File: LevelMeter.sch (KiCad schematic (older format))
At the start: 28 parts, among them U10 NJM4580CG, U8 NJM4580CG, U9 NJM4580CG

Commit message: 改版中
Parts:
- removed C32, C33, C34: 0.1u, Capacitor_SMD:C_0603_1608Metric_Pad1.05x0.95mm_HandSolder, symbol Device:C_Small
- removed C35, C47: 0.47u, Capacitor_THT:CP_Radial_D5.0mm_P2.00mm, symbol Device:CP_Small
- removed C48, C49: option_footprint, Capacitor_SMD:C_0603_1608Metric_Pad1.05x0.95mm_HandSolder, symbol Device:C_Small
- removed D10, D12: SS2040, Diode_SMD:D_SOD-123, symbol Device:D
- removed D11, D13: LED_RED, LED_SMD:LED_0603_1608Metric_Pad1.05x0.95mm_HandSolder, symbol Device:LED
- removed R24: 470k, Resistor_SMD:R_0603_1608Metric_Pad1.05x0.95mm_HandSolder, symbol Device:R_Small
- removed R36: 470, Resistor_SMD:R_0603_1608Metric_Pad1.05x0.95mm_HandSolder, symbol Device:R_Small
- removed unit 3 of U10
- removed unit 2 of U9
- removed unit 1 of U9
- added D10: LED_ORANGE, LED_SMD:LED_0603_1608Metric_Pad1.05x0.95mm_HandSolder, symbol Device:LED
- added D13, D14: 1N4148, Diode_SMD:D_SOD-123, symbol Device:D
- added R23: 1.2k, Resistor_SMD:R_0603_1608Metric_Pad1.05x0.95mm_HandSolder, symbol Device:R_Small
- D8, D9: value SS2040 -> 1N4148
- R21: value 470k -> 22k
- R31: value 4.7k -> 22k
- R32: value 4.7k -> 1.2k
- R35: value 470 -> 1k
- renumbered U10 to U9
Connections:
- wire segments 125 -> 71
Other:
- note added: "-10dBV"
- note removed: "220ms"
- note removed: "Peak\n1/2 Vcc"
- moved on the sheet: C26, C27, C28, C29, C30, C31, R31, R32, R35, U8C, U9A, U9B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

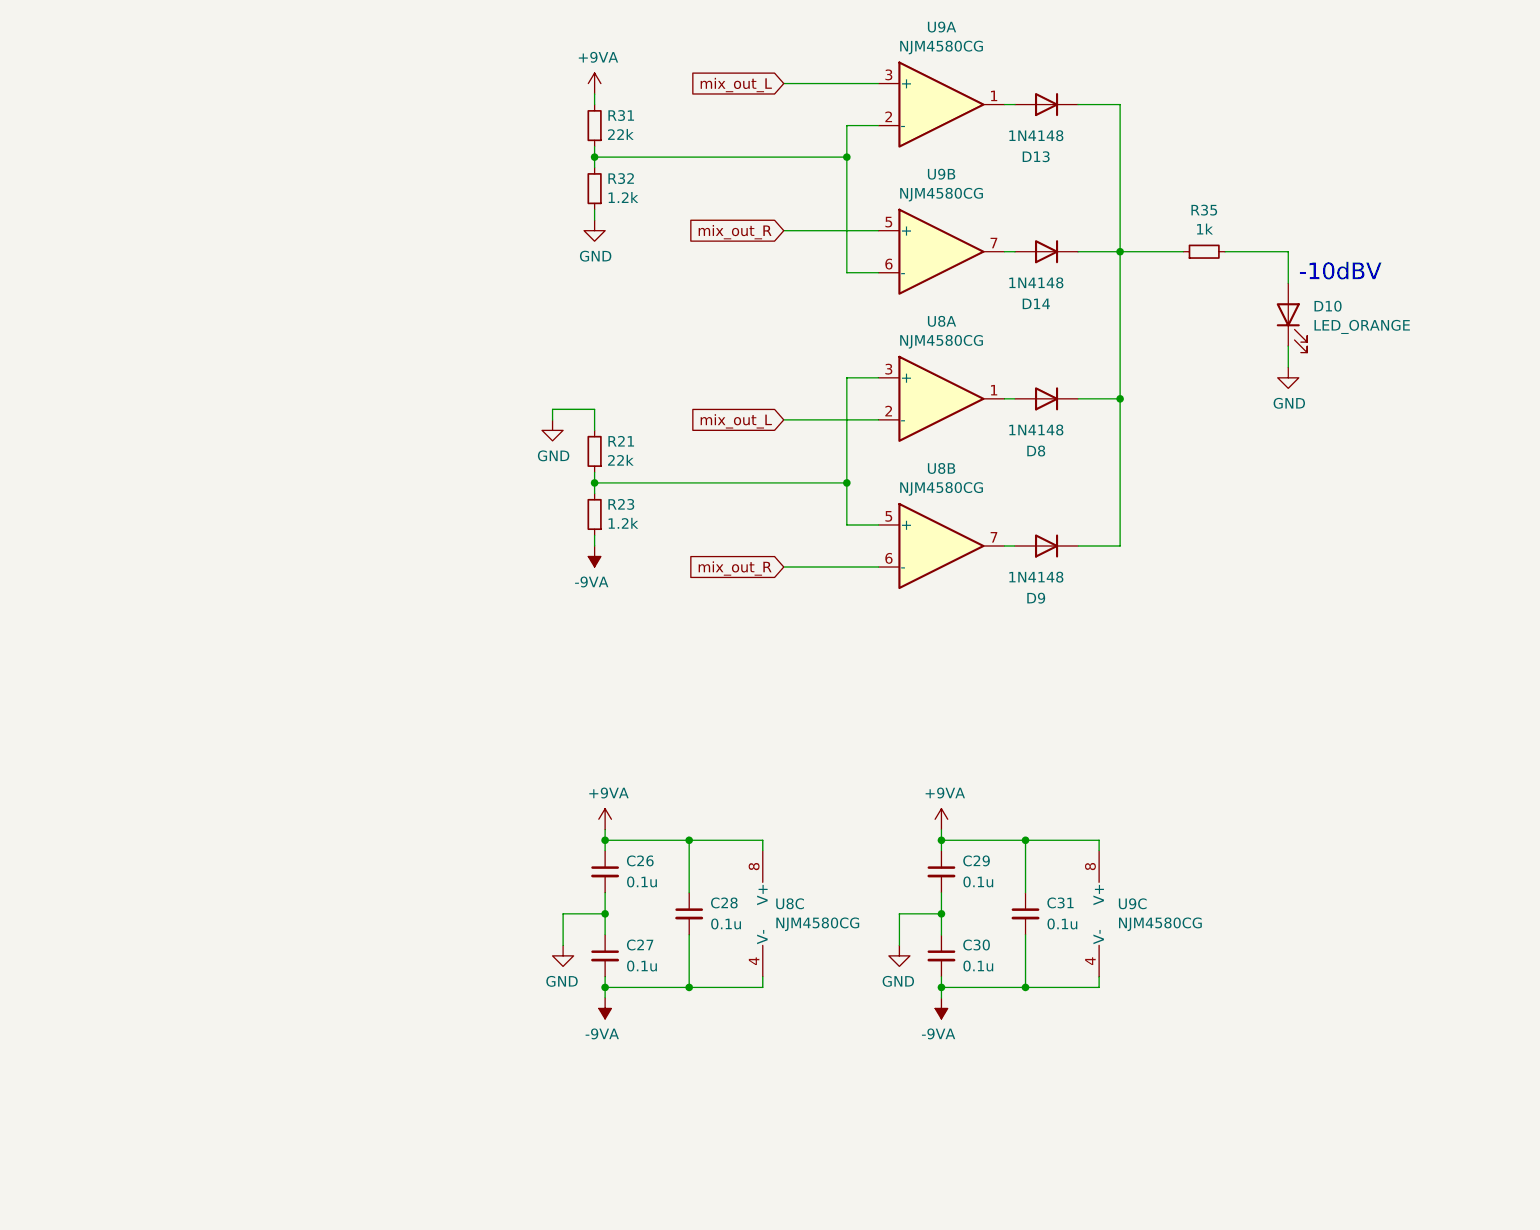
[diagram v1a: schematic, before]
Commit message: Rev.A 作成中
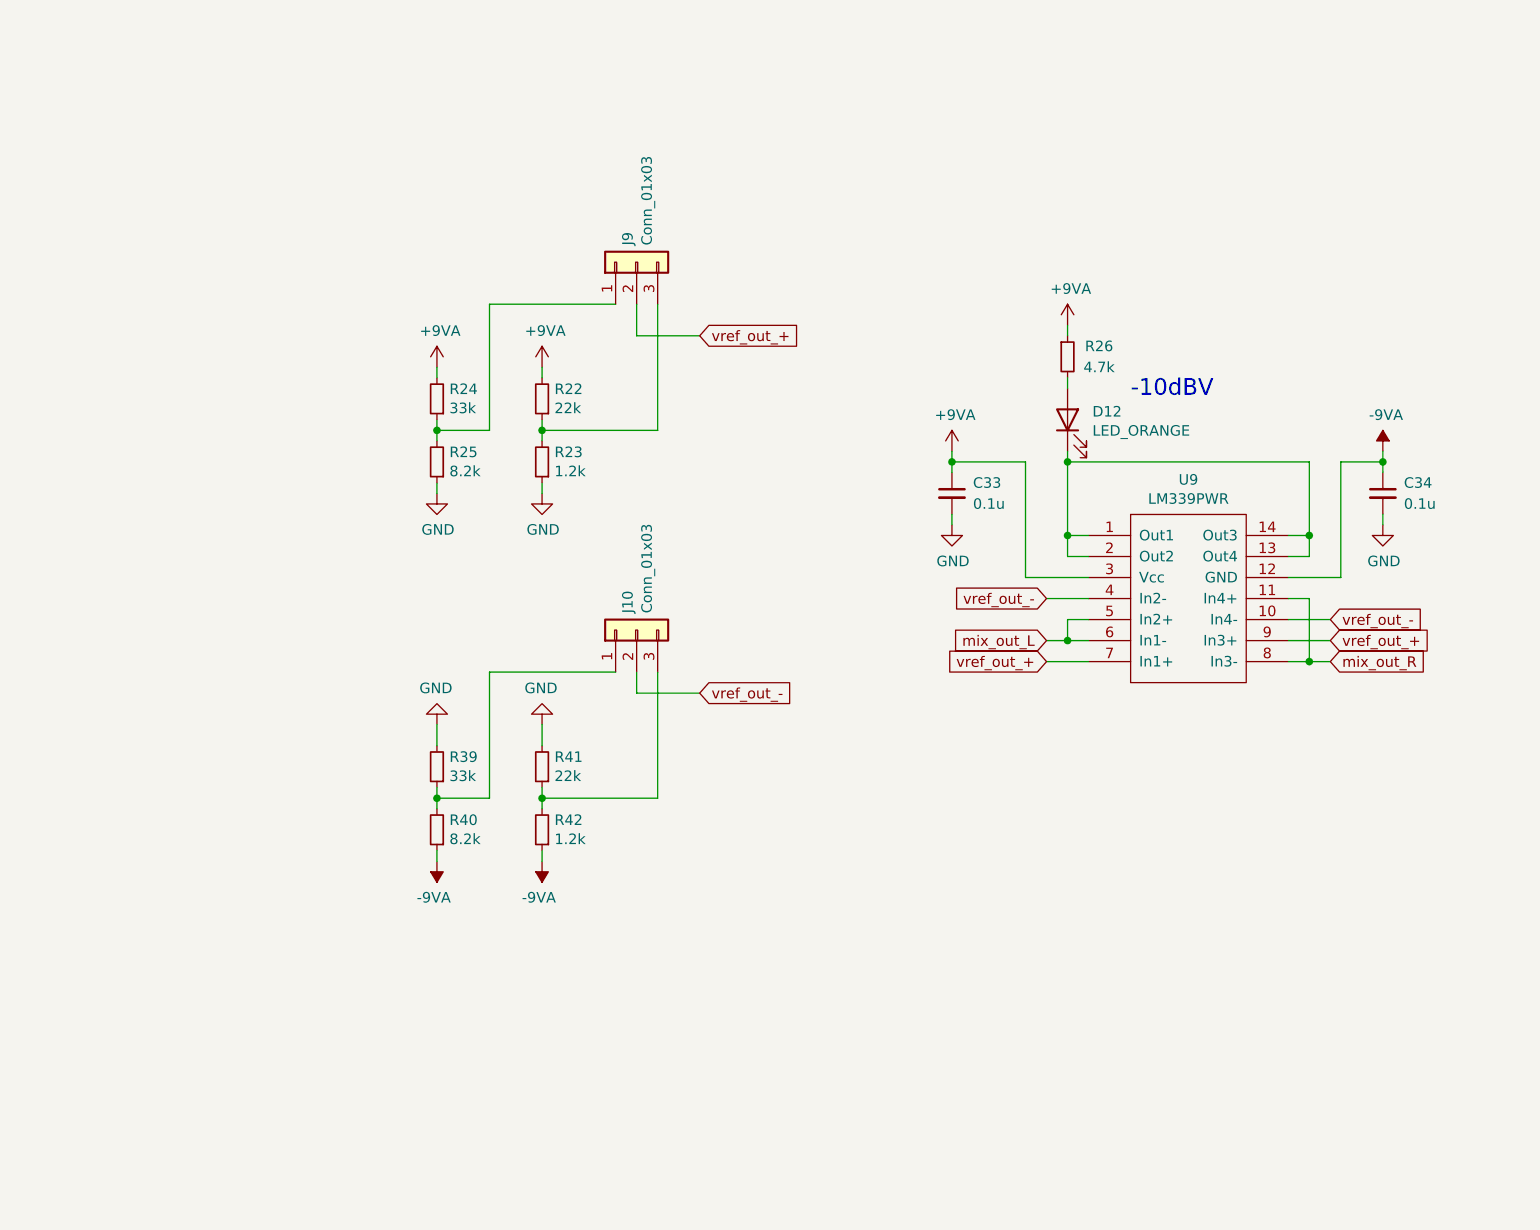
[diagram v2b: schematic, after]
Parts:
- removed C26, C27, C28, C29, C30, C31: 0.1u, Capacitor_SMD:C_0603_1608Metric_Pad1.05x0.95mm_HandSolder, symbol Device:C_Small
- removed D13, D14, D8, D9: 1N4148, Diode_SMD:D_SOD-123, symbol Device:D
- removed R21: 22k, Resistor_SMD:R_0603_1608Metric_Pad1.05x0.95mm_HandSolder, symbol Device:R_Small
- removed R23: 1.2k, Resistor_SMD:R_0603_1608Metric_Pad1.05x0.95mm_HandSolder, symbol Device:R_Small
- removed U8, U9: NJM4580CG, Package_SO:SOP-8_3.9x4.9mm_P1.27mm, symbol Amplifier_Operational:NJM4558
- added C33, C34: 0.1u, Capacitor_SMD:C_0603_1608Metric_Pad1.05x0.95mm_HandSolder, symbol Device:C_Small
- added J10, J9: Conn_01x03, Connector_PinSocket_2.54mm:PinSocket_1x03_P2.54mm_Vertical, symbol Connector_Generic:Conn_01x03
- added R24, R39: 33k, Resistor_SMD:R_0603_1608Metric_Pad1.05x0.95mm_HandSolder, symbol Device:R_Small
- added R25, R40: 8.2k, Resistor_SMD:R_0603_1608Metric_Pad1.05x0.95mm_HandSolder, symbol Device:R_Small
- added R41: 22k, Resistor_SMD:R_0603_1608Metric_Pad1.05x0.95mm_HandSolder, symbol Device:R_Small
- added R42: 1.2k, Resistor_SMD:R_0603_1608Metric_Pad1.05x0.95mm_HandSolder, symbol Device:R_Small
- added U9: LM339PWR, Package_SO:TSSOP-14_4.4x5mm_P0.65mm, symbol toripoyo:LM339PWR
- R26: renamed from R35; value 1k -> 4.7k
- renumbered D10 to D12, R31 to R22, R32 to R23
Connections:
- net +9VA: now also R26.1, C33.1, R24.2, U9.3 (Vcc)
- net -9VA: now also C34.1, R40.1, R42.1, U9.12 (GND)
- net GND: now also C33.2, C34.2, R25.1, R39.2, R41.2; no longer D12.1 (K)
- net mix_out_L: now also U9.5 (In2+), U9.6 (In1-)
- net mix_out_R: now also U9.11 (In4+), U9.8 (In3-)
- net at R22.1, R23.2: now also J9.3 (Pin_3)
- new net: J9.1 (Pin_1), R24.1, R25.2
- new net: J10.3 (Pin_3), R41.1, R42.2
- new net: J10.1 (Pin_1), R39.1, R40.2
- new net: D12.1 (K), U9.1 (Out1), U9.13 (Out4), U9.14 (Out3), U9.2 (Out2)
- new net vref_out_+: J9.2 (Pin_2), U9.7 (In1+), U9.9 (In3+)
- new net vref_out_-: J10.2 (Pin_2), U9.10 (In4-), U9.4 (In2-)
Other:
- moved on the sheet: D12, R22, R23, R26
